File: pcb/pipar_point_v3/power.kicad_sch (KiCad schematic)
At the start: 32 parts, among them IC1 MCP1700T-3302E_MAY, J1 USB_C_Receptacle_USB2.0_16P, J5 Conn_01x02, SW3 SW_SPDT, U11 nPM1300-QEXX, U3 MAX17048, U4 ESDR0502NMUTAG, U5 nPM1100-QDXX

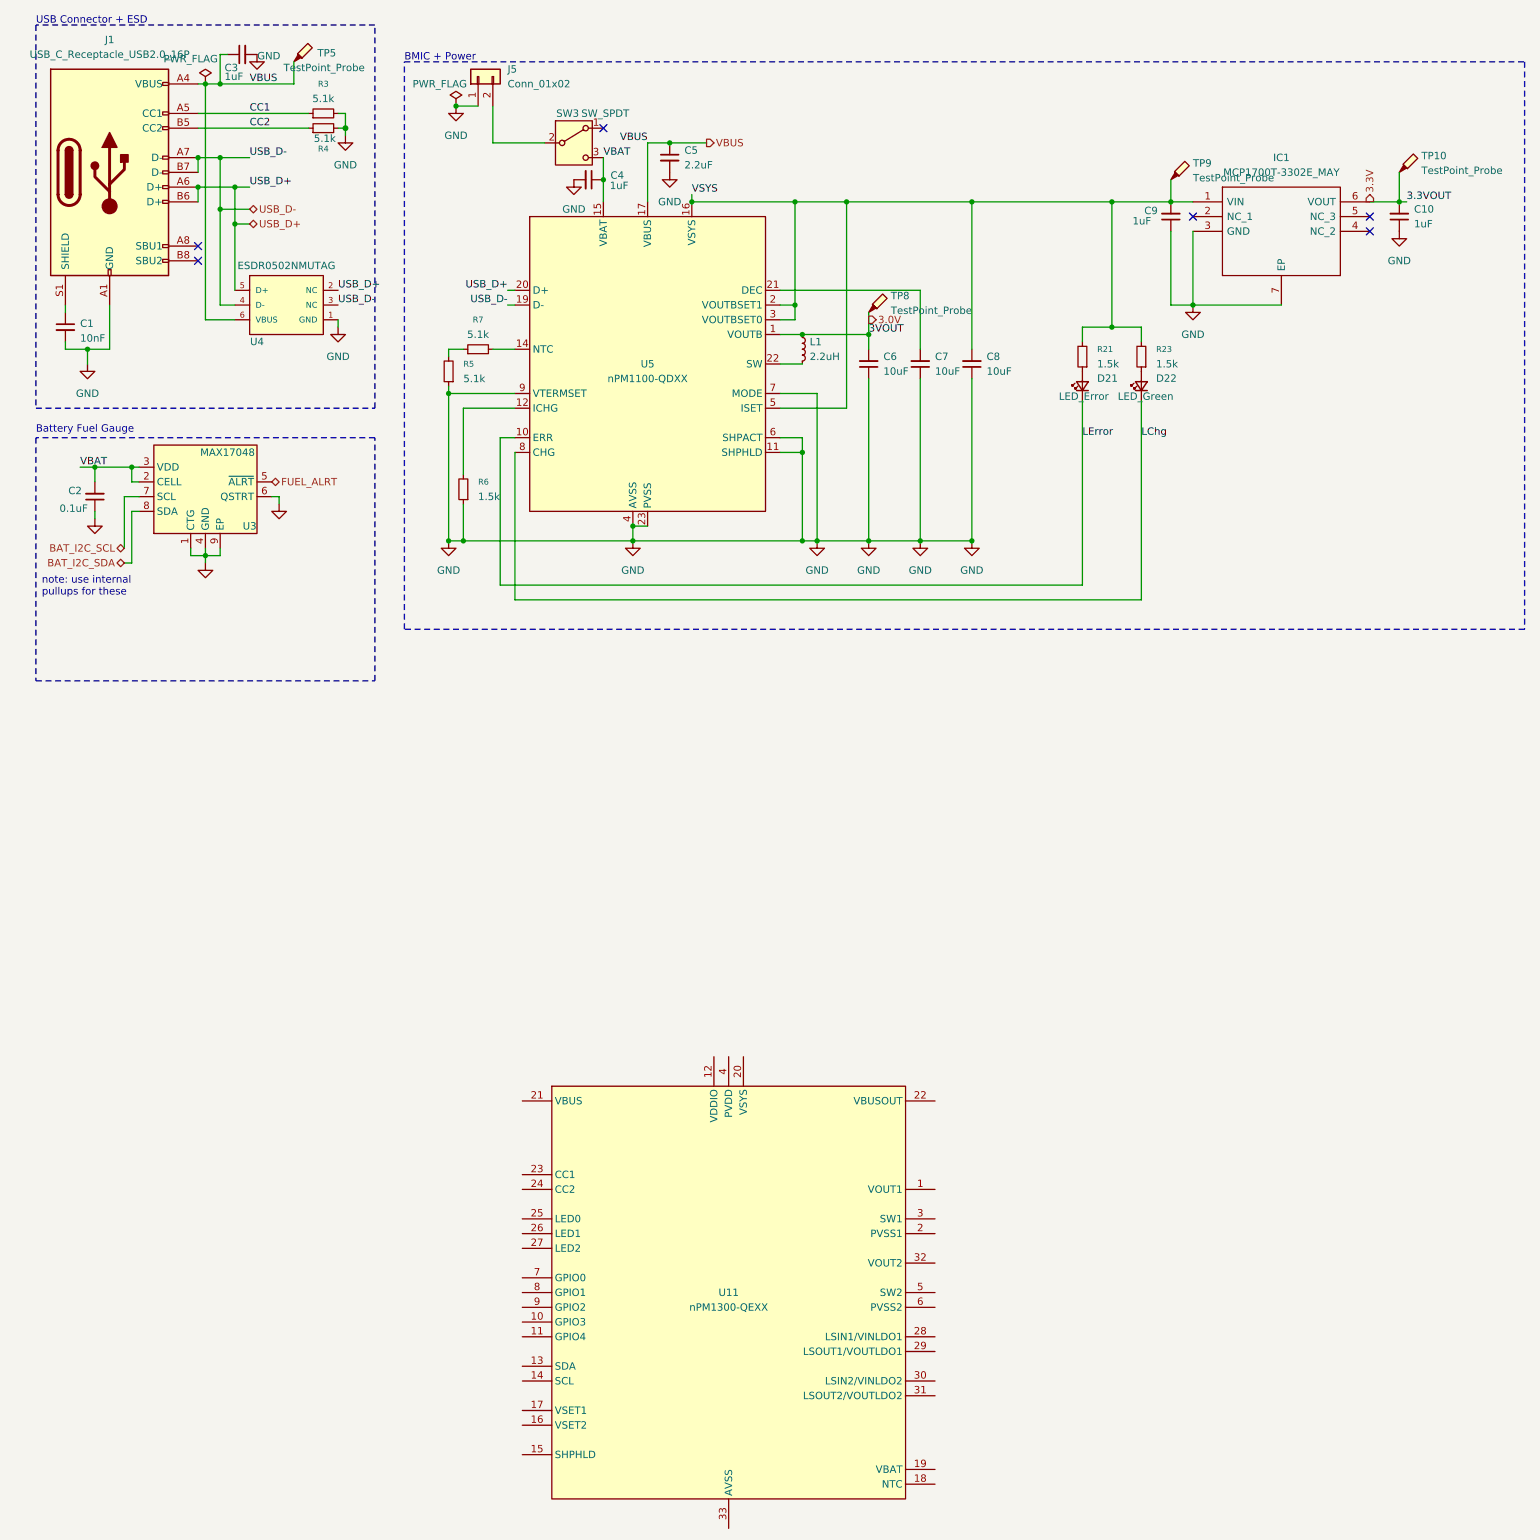
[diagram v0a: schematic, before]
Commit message: changed npm1100 to npm1300 and got rid of some footprints
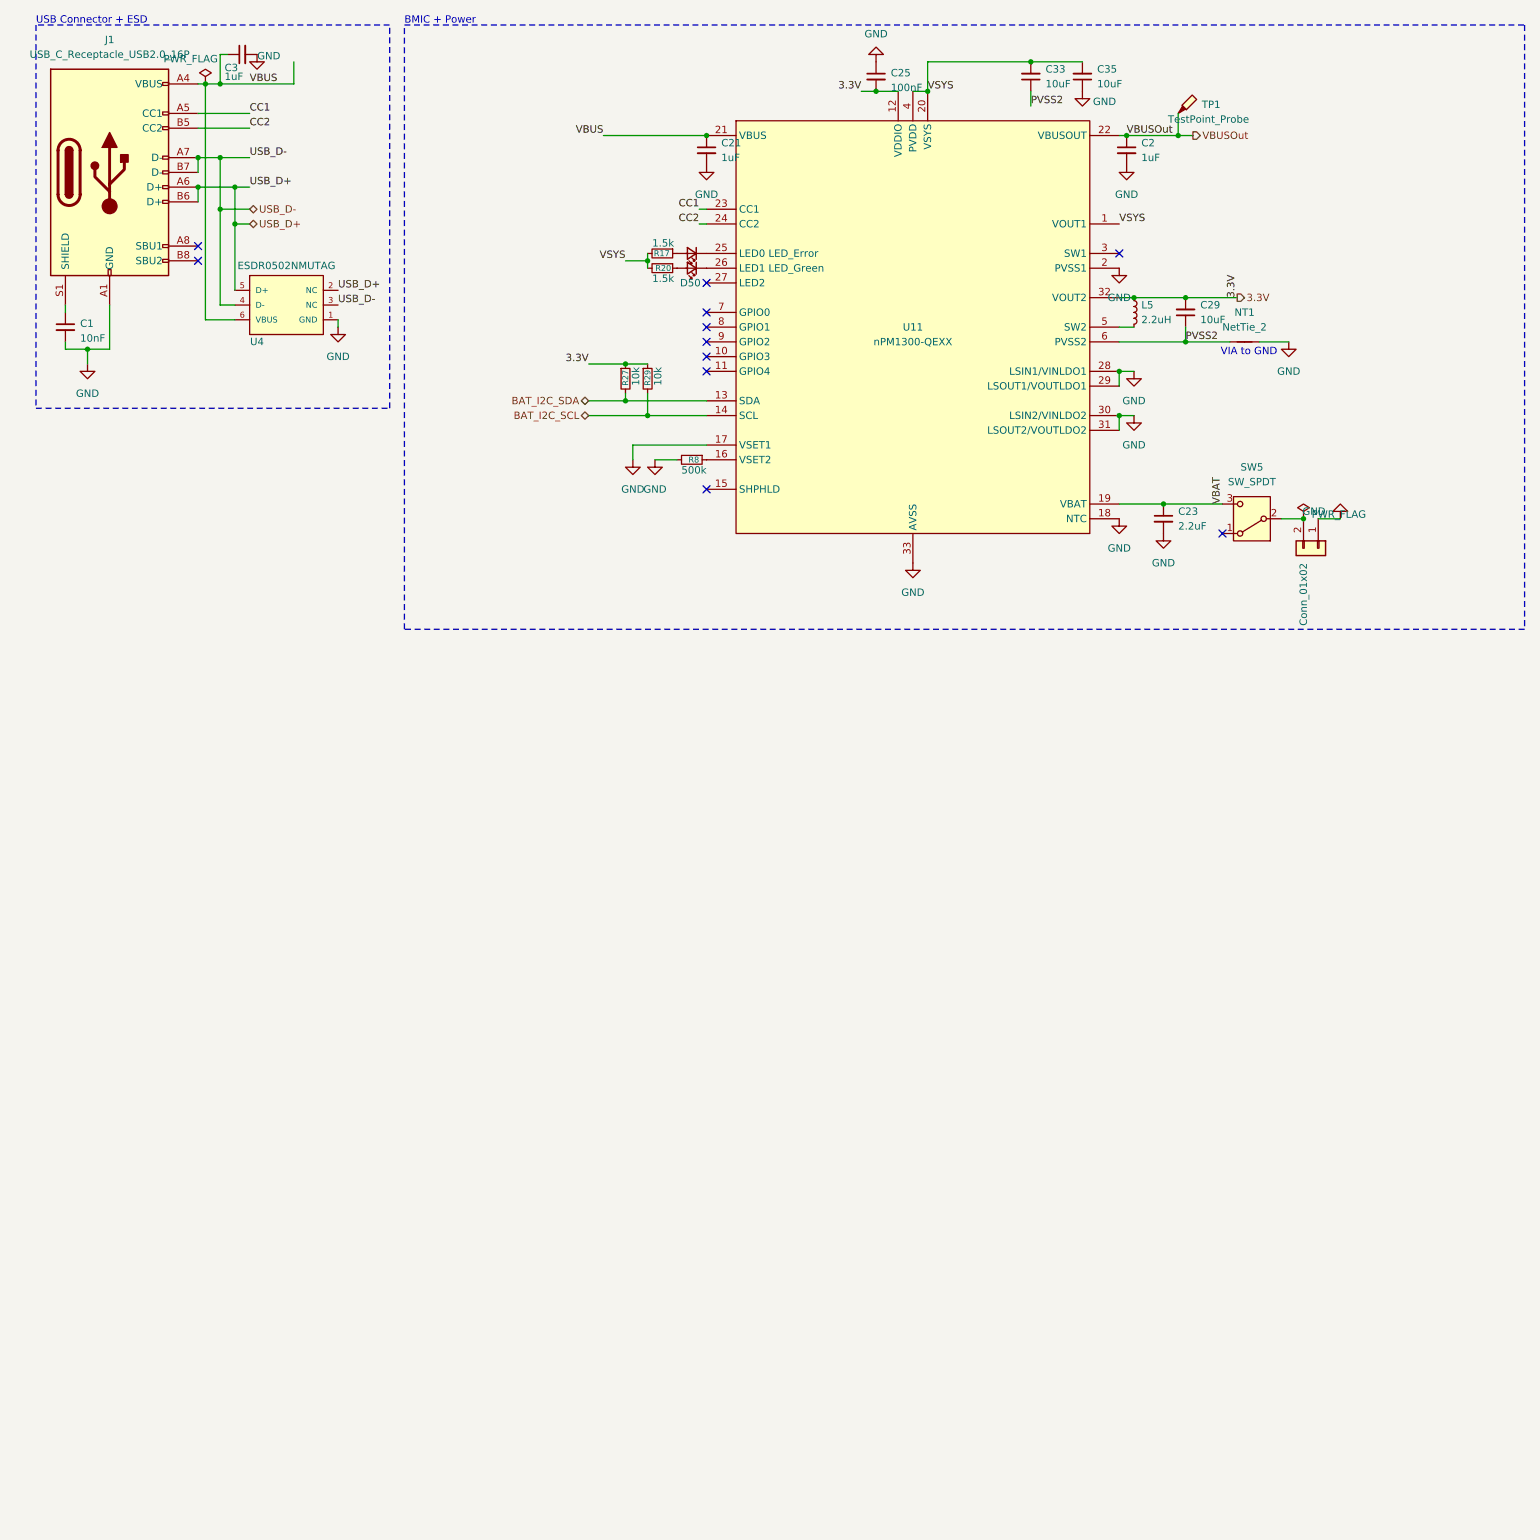
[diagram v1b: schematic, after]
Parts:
- removed C10, C4, C9: 1uF, Capacitor_SMD:C_0603_1608Metric, symbol Device:C_Small
- removed C5: 2.2uF, Capacitor_SMD:C_0603_1608Metric, symbol Device:C_Small
- removed C6, C7, C8: 10uF, Capacitor_SMD:C_0603_1608Metric, symbol Device:C_Small
- removed D21: LED_Error, LED_SMD:LED_0603_1608Metric, symbol Device:LED_Small
- removed D22: LED_Green, LED_SMD:LED_0603_1608Metric, symbol Device:LED_Small
- removed IC1: MCP1700T-3302E_MAY, SamacSys_Parts:SON65P200X200X90-7N, symbol SamacSys_Parts:MCP1700T-3302E_MAY
- removed L1: 2.2uH, Inductor_SMD:L_0805_2012Metric, symbol Device:L_Small
- removed R21, R23, R6: 1.5k, Resistor_SMD:R_0603_1608Metric, symbol Device:R_Small
- removed R3, R4, R5, R7: 5.1k, Resistor_SMD:R_0603_1608Metric, symbol Device:R_Small
- removed SW3: SW_SPDT, Button_Switch_SMD:SW_SPDT_PCM12, symbol Switch:SW_SPDT
- removed TP10, TP5, TP8, TP9: TestPoint_Probe, TestPoint:TestPoint_Pad_D1.0mm, symbol Connector:TestPoint_Probe
- removed U3: MAX17048, Package_DFN_QFN:TDFN-8-1EP_2x2mm_P0.5mm_EP0.8x1.2mm, symbol mikoto:MAX17048
- removed U5: nPM1100-QDXX, Package_DFN_QFN:QFN-24-1EP_4x4mm_P0.5mm_EP2.6x2.6mm_ThermalVias, symbol PCM_nordic-lib-kicad-npm:nPM1100-QDXX
- added C21: 1uF, Capacitor_SMD:C_0603_1608Metric, symbol Device:C_Small
- added C23: 2.2uF, Capacitor_SMD:C_0603_1608Metric, symbol Device:C_Small
- added C25: 100nF, Capacitor_SMD:C_0603_1608Metric, symbol Device:C_Small
- added C29, C33, C35: 10uF, Capacitor_SMD:C_0603_1608Metric, symbol Device:C_Small
- added D47: LED_Error, LED_SMD:LED_0603_1608Metric, symbol Device:LED_Small
- added D50: LED_Green, LED_SMD:LED_0603_1608Metric, symbol Device:LED_Small
- added L5: 2.2uH, Inductor_SMD:L_0805_2012Metric, symbol Device:L_Small
- added NT1: NetTie_2, NetTie:NetTie-2_THT_Pad0.3mm, symbol Device:NetTie_2
- added R17, R20: 1.5k, Resistor_SMD:R_0603_1608Metric, symbol Device:R_Small
- added R27, R29: 10k, Resistor_SMD:R_0603_1608Metric, symbol Device:R_Small
- added R8: 500k, Resistor_SMD:R_0603_1608Metric, symbol Device:R_Small
- added SW5: SW_SPDT, Button_Switch_SMD:SW_SPDT_PCM12, symbol Switch:SW_SPDT
- added TP1: TestPoint_Probe, TestPoint:TestPoint_Pad_D1.0mm, symbol Connector:TestPoint_Probe
- C2: value 0.1uF -> 1uF; Manufacturer_Part_Number C1608X7R1H104K080AA -> LMK107B7105KA-T; Mouser Part Number 810-C1608X7R1H104K -> 963-LMK107B7105KA-T
- C3: Manufacturer_Part_Number CGA3E1X7R1V105K080AC -> LMK107B7105KA-T; Mouser Part Number 810-CGA3E1X7R1V105KC -> 963-LMK107B7105KA-T
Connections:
- net 3.3V: now also U11.12 (VDDIO), U11.32 (VOUT2), C25.2, C29.2, L5.1, R27.1, R29.1
- net BAT_I2C_SCL: now also U11.14 (SCL), R29.2
- net BAT_I2C_SDA: now also U11.13 (SDA), R27.2
- net CC1: now also U11.23 (CC1)
- net CC2: now also U11.24 (CC2)
- net GND: now also C2.2, U11.17 (VSET1), U11.18 (NTC), U11.2 (PVSS1), U11.28 (LSIN1/VINLDO1), U11.29 (LSOUT1/VOUTLDO1), U11.30 (LSIN2/VINLDO2), U11.31 (LSOUT2/VOUTLDO2), U11.33 (AVSS), C21.2, C23.2, C25.1, C35.1, NT1.2, R8.2; no longer C2.1
- net VBAT: now also U11.19 (VBAT), C23.1, SW5.3 (C); no longer C2.2
- net VBUS: now also U11.21 (VBUS), C21.1
- net VSYS: now also U11.1 (VOUT1), U11.20 (VSYS), U11.4 (PVDD), C33.2, C35.2, R17.2, R20.2
- net at U11.16 (VSET2): now also R8.1
- net VBUSOut: now reaches U11.22 (VBUSOUT)
- net VBUSOut: now also C2.1, TP1.1
- net at U11.25 (LED0): now also D47.1 (K)
- net at U11.26 (LED1): now also D50.1 (K)
- net at U11.5 (SW2): now also L5.2
- net PVSS2: now reaches U11.6 (PVSS2)
- net PVSS2: now also C29.1, C33.1, NT1.1
- net at J5.2 (Pin_2): now also SW5.2 (B)
- new net: D50.2 (A), R20.1
- new net: D47.2 (A), R17.1
- no-connect marks 6 -> 11
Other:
- note added: "VIA to GND"
- note removed: "Battery Fuel Gauge"
- note removed: "note: use internal pullups for these"
- moved on the sheet: U11
